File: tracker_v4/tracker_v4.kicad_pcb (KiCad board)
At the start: 2 copper layers, 62.5 x 22.1 mm, 36 parts, among them J1 USB_C_Receptacle_PowerOnly_6P, J2 P70-7000045, J3 P70-7000045, Q1 DMG9926UDM-7, U1 XIAO-ESP32-DIP, U2 LIS3DH, U3 DW01A, U4 INA226AIDGSR, U5 TP4056-42-ESOP8

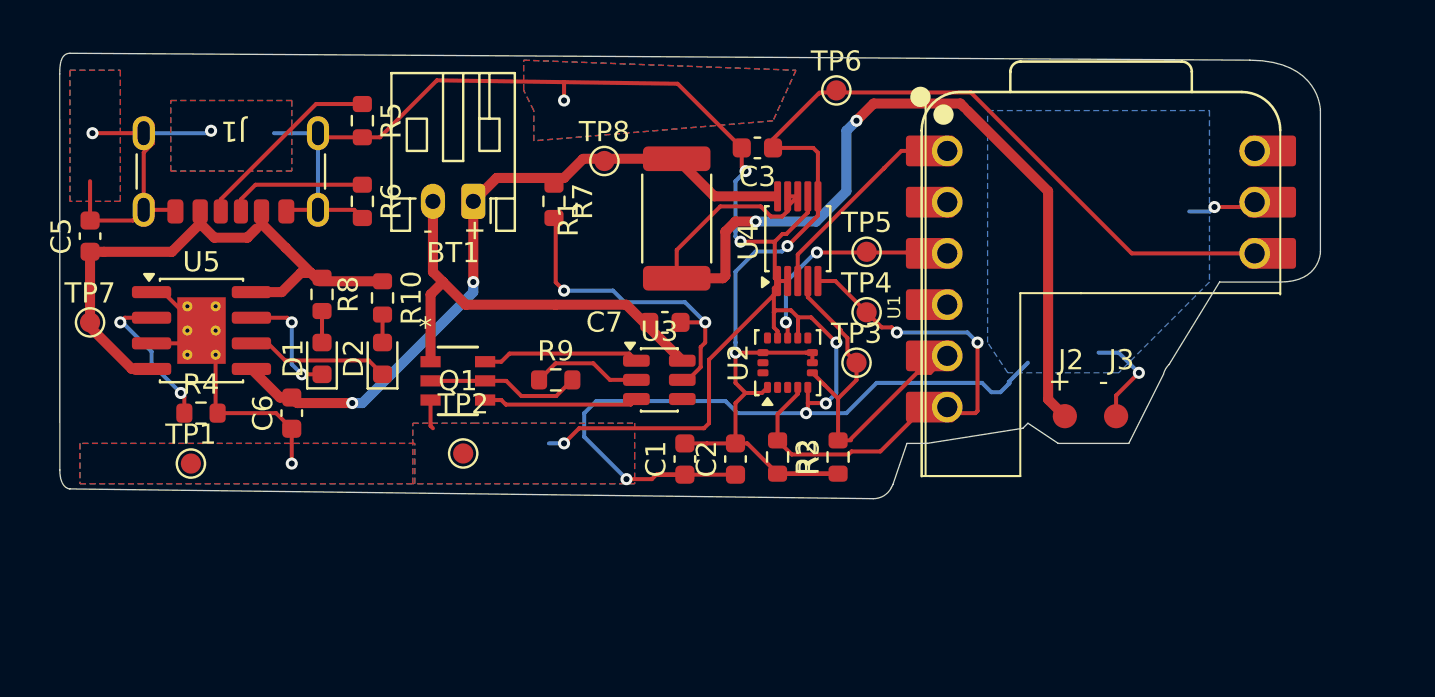
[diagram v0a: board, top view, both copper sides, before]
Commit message: started pcb v4
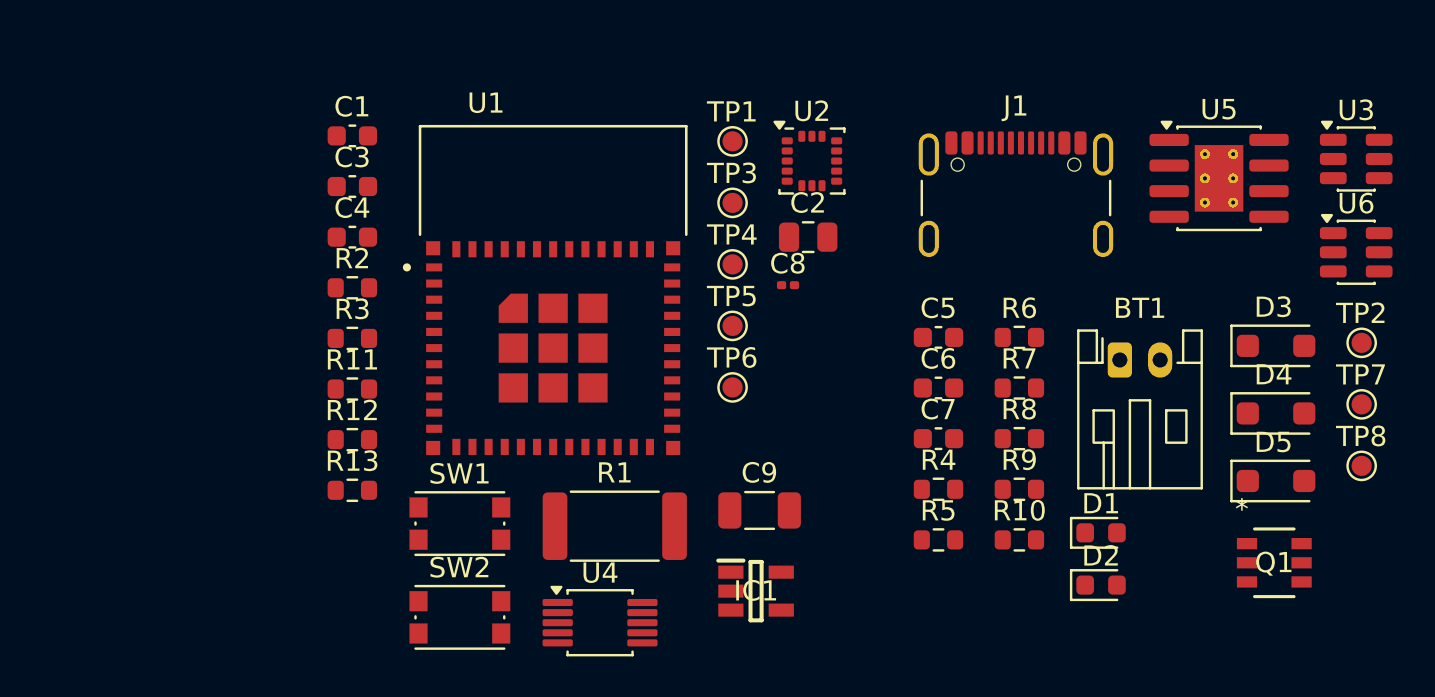
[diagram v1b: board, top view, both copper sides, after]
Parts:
- removed J2, J3: P70-7000045, P70_7000045:HARWIN_P70-7000045
- added C4: 1u, Capacitor_SMD:C_0603_1608Metric, F.Cu at (146.0, 81.3)
- added C8: 10u, Capacitor_SMD:C_0201_0603Metric, F.Cu at (167.6, 83.7)
- added C9: 22u, Capacitor_SMD:C_1206_3216Metric, F.Cu at (166.2, 94.8)
- added D3: D, Diode_SMD:D_SOD-123F, F.Cu at (191.8, 86.7)
- added D4: D, Diode_SMD:D_SOD-123F, F.Cu at (191.8, 90.0)
- added D5: D, Diode_SMD:D_SOD-123F, F.Cu at (191.8, 93.4)
- added IC1: RT9080-33GJ5, RT9080-33GJ5:SOT94P280X100-5N, F.Cu at (166.0, 98.8)
- added R11: 10k, Resistor_SMD:R_0603_1608Metric, F.Cu at (146.0, 88.8)
- added R12: 10k, Resistor_SMD:R_0603_1608Metric, F.Cu at (146.0, 91.3)
- added R13: 4.7k, Resistor_SMD:R_0603_1608Metric, F.Cu at (146.0, 93.8)
- added SW1: SW_Push, Button_Switch_SMD:SW_Push_1P1T_NO_CK_KMR2, F.Cu at (151.3, 95.5)
- added SW2: SW_Push, Button_Switch_SMD:SW_Push_1P1T_NO_CK_KMR2, F.Cu at (151.3, 100.1)
- added U6: USBLC6-2SC6, Package_TO_SOT_SMD:SOT-23-6, F.Cu at (195.8, 82.0)
- C2: footprint Capacitor_SMD:C_0603_1608Metric -> Capacitor_SMD:C_0805_2012Metric
- J1: value USB_C_Receptacle_PowerOnly_6P -> USB_C_Receptacle_USB2.0_16P; footprint Connector_USB:USB_C_Receptacle_GCT_USB4125-xx-x-0190_6P_TopMnt_Horizontal -> Connector_USB:USB_C_Receptacle_GCT_USB4105-xx-A_16P_TopMnt_Horizontal
- R4: value 1.2k -> 3.0k
- U1: value XIAO-ESP32-DIP -> ESP32-C6-MINI-1-N4; footprint Seeed_Studio_XIAO_Series:XIAO-ESP32-C6-DIP -> ESP32-C6-MINI-1-N4:XCVR_ESP32-C6-MINI-1-N4
- moved TP7 63.2 mm to (196.0, 89.6)
- moved U5 51.0 mm to (189.0, 78.4)
- moved TP2 44.9 mm to (196.0, 86.5)
- moved C5 42.4 mm to (175.1, 86.2), turned to 0 degrees
- moved Q1 41.5 mm to (191.7, 97.4)
- moved TP8 40.5 mm to (196.0, 92.6)
- moved D1 39.6 mm to (183.1, 95.9), turned to 0 degrees
- moved J1 39.1 mm to (178.9, 80.3), turned to 0 degrees
- moved D2 37.4 mm to (183.1, 98.5), turned to 0 degrees
- moved R4 36.8 mm to (175.1, 93.8)
- moved U3 36.2 mm to (195.8, 77.4)
- moved R5 35.3 mm to (175.1, 96.3), turned to 0 degrees
- moved R8 35.3 mm to (179.1, 91.3), turned to 0 degrees
- moved R10 33.8 mm to (179.1, 96.3), turned to 0 degrees
- moved R6 33.3 mm to (179.1, 86.2), turned to 0 degrees
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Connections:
- net /Shunt_Output renamed SHUNT_OUTPUT
- C5 pad 2: GND -> Net-(D4-A)
- J1 pad B5: Net-(J1-CC2) -> USB_DM
- R5 pad 1: Net-(J1-CC2) -> USB_DM
- R5 pad 2: GND -> Net-(D3-A)
- R6 pad 2: GND -> Net-(D5-A)
- TP5 pad 1: Net-(U1-D2) -> 3v3
- U1 pad 1: Net-(U1-D0) -> GND
- U1 pad 12: 3v3 -> INA226_ALERT
- U1 pad 13: GND -> unconnected-(U1-IO1-Pad13)
- U1 pad 14: unconnected-(U1-VBUS-Pad14)_1 -> GND
- U1 pad 2: unconnected-(U1-D1-Pad2)_1 -> GND
- U1 pad 3: Net-(U1-D2) -> 3v3
- U1 pad 5: SDA -> LIS3DH_INT1
- U1 pad 6: SCL -> unconnected-(U1-IO3-Pad6)
- U2 pad 11: Net-(U1-D2) -> LIS3DH_INT1
- U4 pad 3: Net-(U1-D0) -> INA226_ALERT
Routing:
- net GND: track 153.3 -> 0.00 mm, vias 13 -> 0
- net 3v3: track 64.9 -> 0.00 mm, vias 2 -> 0
- net SHUNT_OUTPUT: track 48.4 -> 0.00 mm, vias 2 -> 0
- net /Charging_and_Battery/BAT+: track 35.4 -> 0.00 mm, vias 2 -> 0
- net USB_VBUS: track 29.2 -> 0.00 mm
- net SCL: track 26.3 -> 0.00 mm, vias 2 -> 0
- net /Charging_and_Battery/BAT-: track 21.9 -> 0.00 mm
- net SDA: track 18.2 -> 0.00 mm
- net Net-(U3-VCC): track 16.0 -> 0.00 mm, vias 2 -> 0
- net Net-(U1-D2): track 11.6 -> 0.00 mm, vias 2 -> 0
- net Net-(U1-D0): track 10.9 -> 0.00 mm
- net Net-(J1-CC2): track 9.58 -> 0.00 mm
- net Net-(U3-OD): track 7.81 -> 0.00 mm
- net Net-(U3-OC): track 7.71 -> 0.00 mm
- net /Charging_and_Battery/PROTECT_MID: track 7.67 -> 0.00 mm
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- removed copper zone on B.Cu, net GND
- removed copper zone on F.Cu, net GND
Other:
- board outline removed
- board text removed: "+"
- board text removed: "-"
